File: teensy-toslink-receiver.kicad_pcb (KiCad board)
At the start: 2 copper layers, 24.9 x 18.3 mm, 17 parts, among them J1 Conn_01x03, J2 Conn_01x05, J3 Conn_01x05, J4 Conn_01x05, J5 Conn_01x03, J6 Conn_01x04, J7 HDMI_A_1.4, Q1 BSS138, Q2 BSS138, Q3 BSS138, U1 PLR135-T10

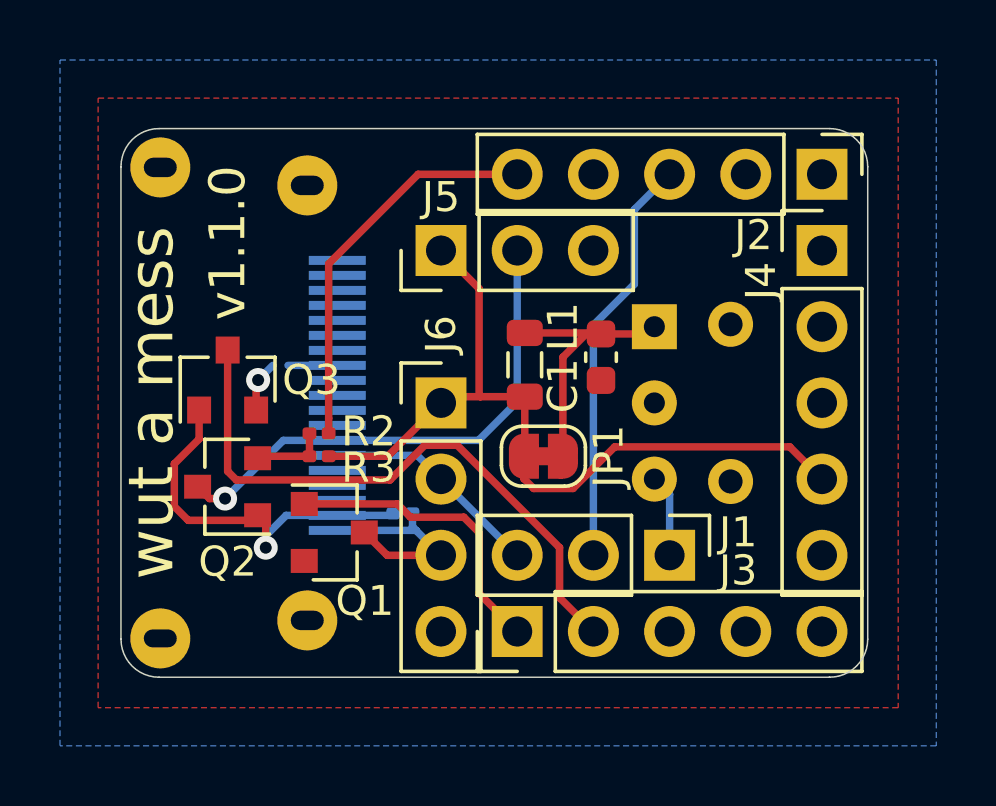
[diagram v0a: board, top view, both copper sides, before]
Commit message: Best-effort automated zone fill conversion
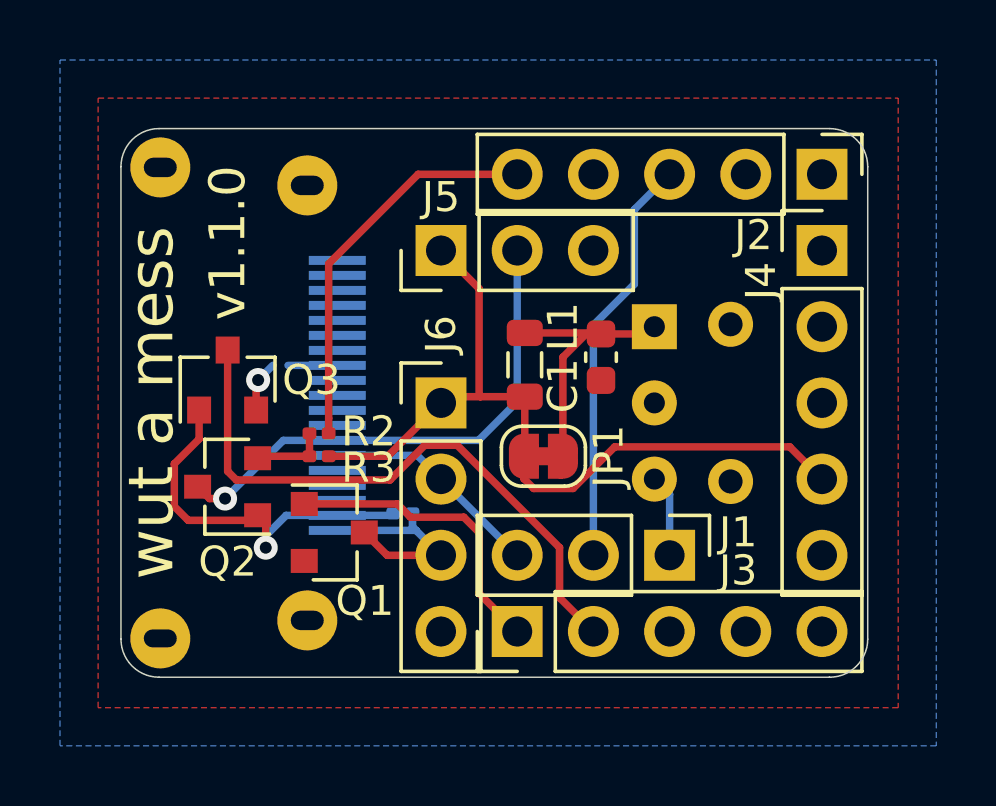
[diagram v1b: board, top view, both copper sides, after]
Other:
- net class Default removed
